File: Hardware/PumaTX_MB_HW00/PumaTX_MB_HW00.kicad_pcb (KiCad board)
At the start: 4 copper layers, 130 x 40 mm, 115 parts, among them J100 FH12A-26S-0.5SH_55_, J101 FH12-12S-0.5SH_55_, J102 500334-0160, J103 500334-0160, J104 692122030100, J105 53398-0667, J400 U.FL-R-SMT-1_40_, J410 U.FL-R-SMT-1_40_, M130 Motor_DC, M140 Fan, Q130 ZXMN3B01F, Q140 ZXMN3B01F, Q200 UMH3NTN, Q201 UMH3NTN, U200 CP2105-F01-GMR, U300 ESP32-PICO-D4, U400 ESP32-PICO-D4, U402 E28-2G4M27S, U410 SX1280, U500 BQ24075RGTR, U510 MIC5528-3.3YMT-T5, U520 MIC5528-3.3YMT-T5, U530 MIC5528-3.3YMT-T5, Y410 NX2016SA-52MHZ-EXS00A-CS06016

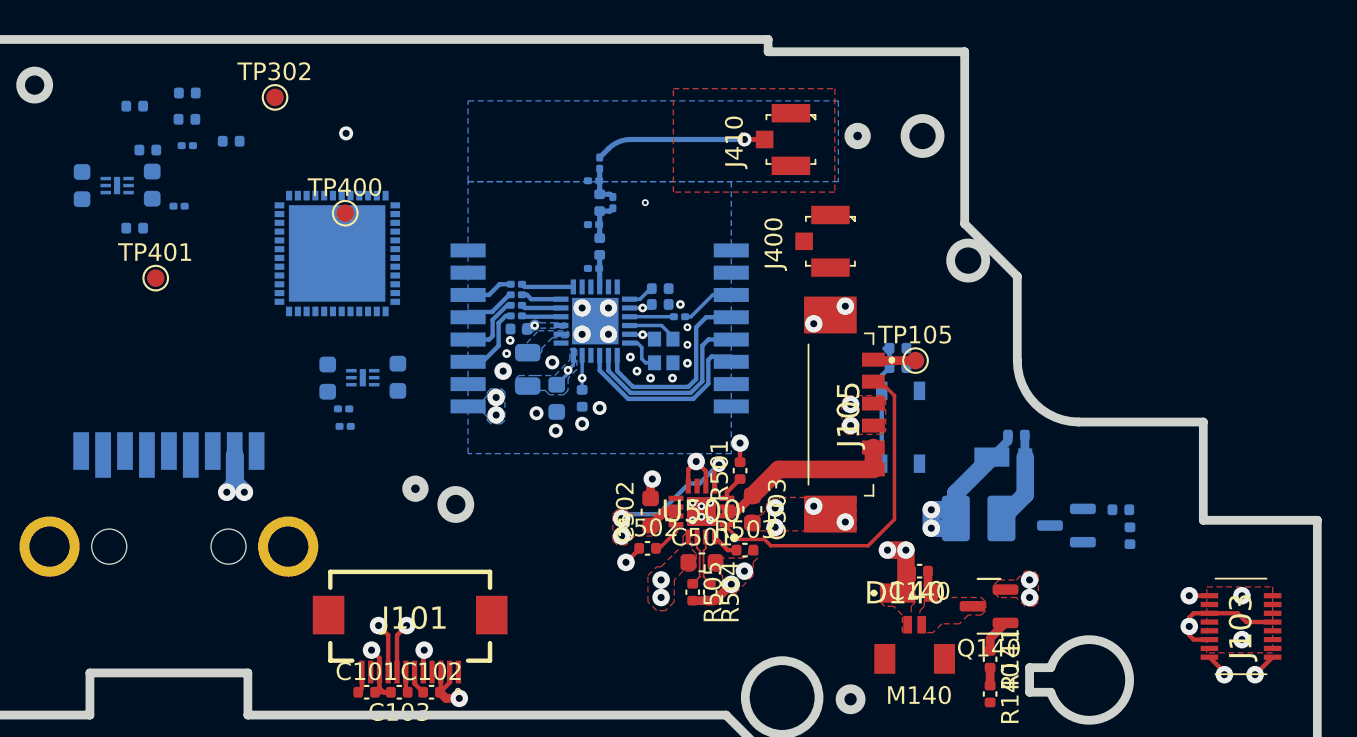
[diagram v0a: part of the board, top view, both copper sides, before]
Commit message: rf backup
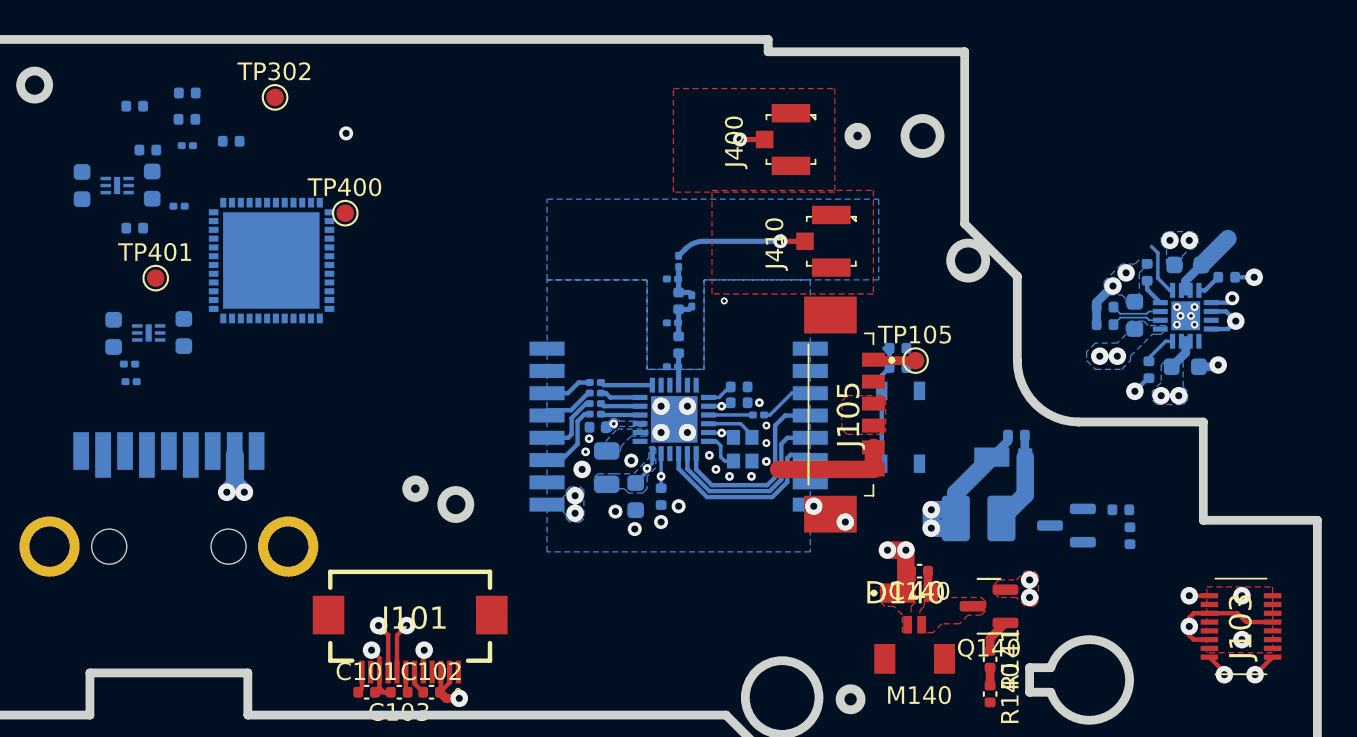
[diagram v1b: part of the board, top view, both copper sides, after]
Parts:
- C501, C502, C503, R501, R502, R503, R504, R505, U500: moved to B.Cu
- moved C502 31.6 mm to (203.9, 101.8), turned to 0 degrees
- moved R502 30.3 mm to (201.8, 102.0), turned to 90 degrees
- moved R501 29.8 mm to (206.2, 96.8), turned to 0 degrees
- moved U500 29.8 mm to (203.9, 99.0), turned to -90 degrees
- moved C503 28.5 mm to (204.0, 96.0), turned to 180 degrees
- moved C501 28.4 mm to (201.0, 98.9), turned to 90 degrees
- moved R505 28.0 mm to (199.3, 99.5), turned to 180 degrees
- moved R503 27.9 mm to (201.7, 96.5), turned to 90 degrees
- moved R504 27.8 mm to (199.3, 98.5), turned to 180 degrees
- moved R512 12.5 mm to (143.8, 102.7)
- moved C530 12.5 mm to (142.8, 100.0)
- moved C531 12.5 mm to (146.8, 99.9)
- moved R511 12.5 mm to (143.7, 101.7)
- moved U530 12.5 mm to (144.8, 99.9)
- moved C416 7.18 mm to (178.4, 103.9)
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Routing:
- net /VSYS: track 52.3 -> 29.3 mm
- net /BATTERY_TEMP: track 19.4 -> 3.18 mm
- net VBUS: track 103.0 -> 99.9 mm
- net /50_ELRS_ANT_4: track 9.88 -> 7.48 mm
- net /50_ESP_ELRS_ANT_2: track 0.00 -> 1.40 mm, vias 0 -> 1
- net GND: vias 65 -> 61
- added copper zone on B.Cu, net /VSYS
- added copper zone on B.Cu, net VBUS
